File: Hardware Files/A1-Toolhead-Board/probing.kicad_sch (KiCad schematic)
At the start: 2 parts, among them J10 BL_PROBE, J9 ADXL345

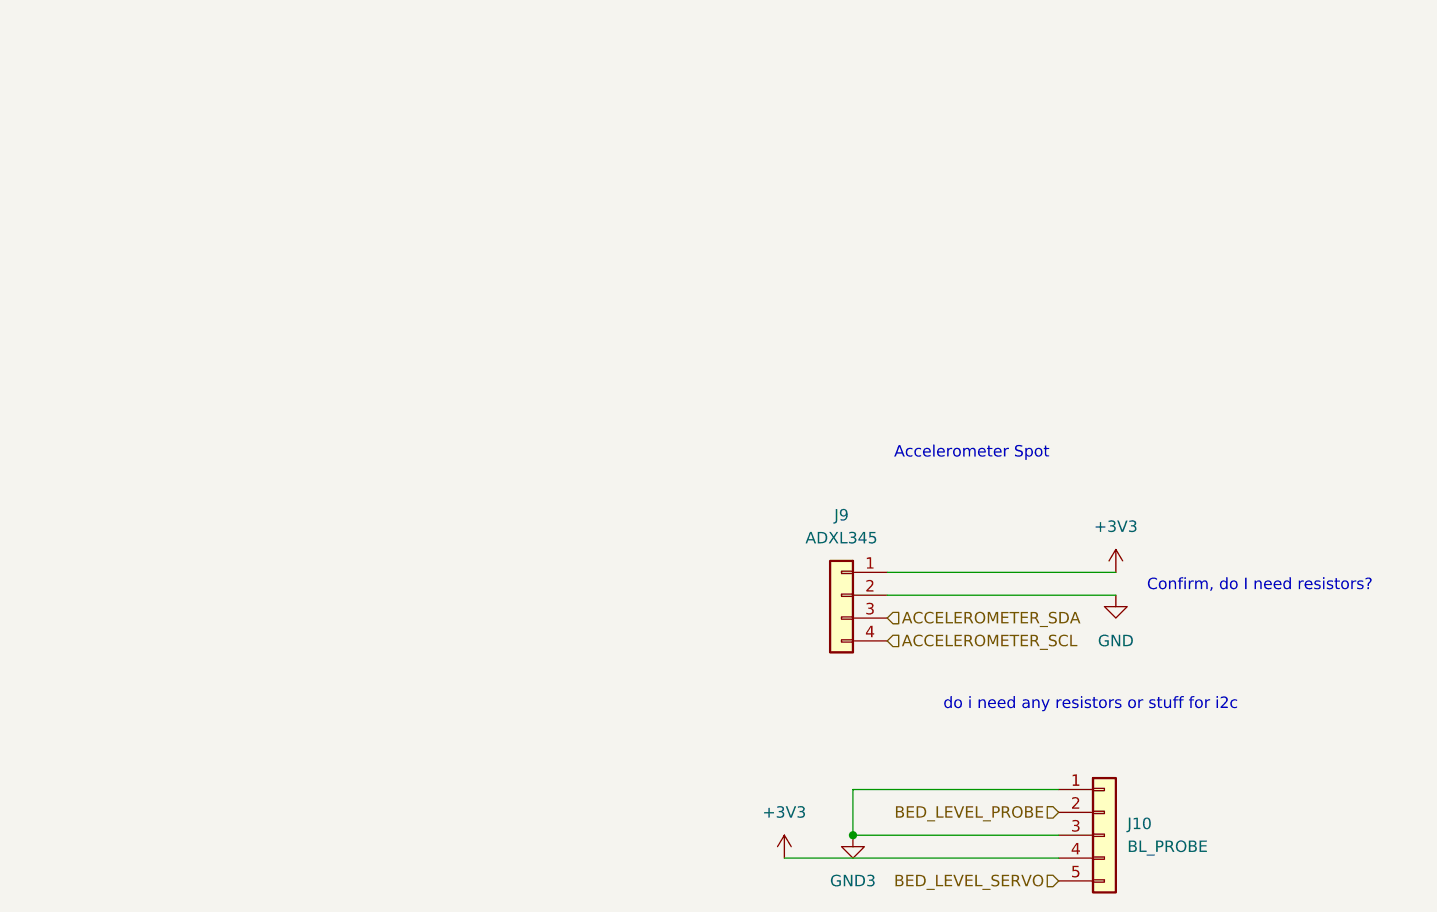
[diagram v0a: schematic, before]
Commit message: e
e
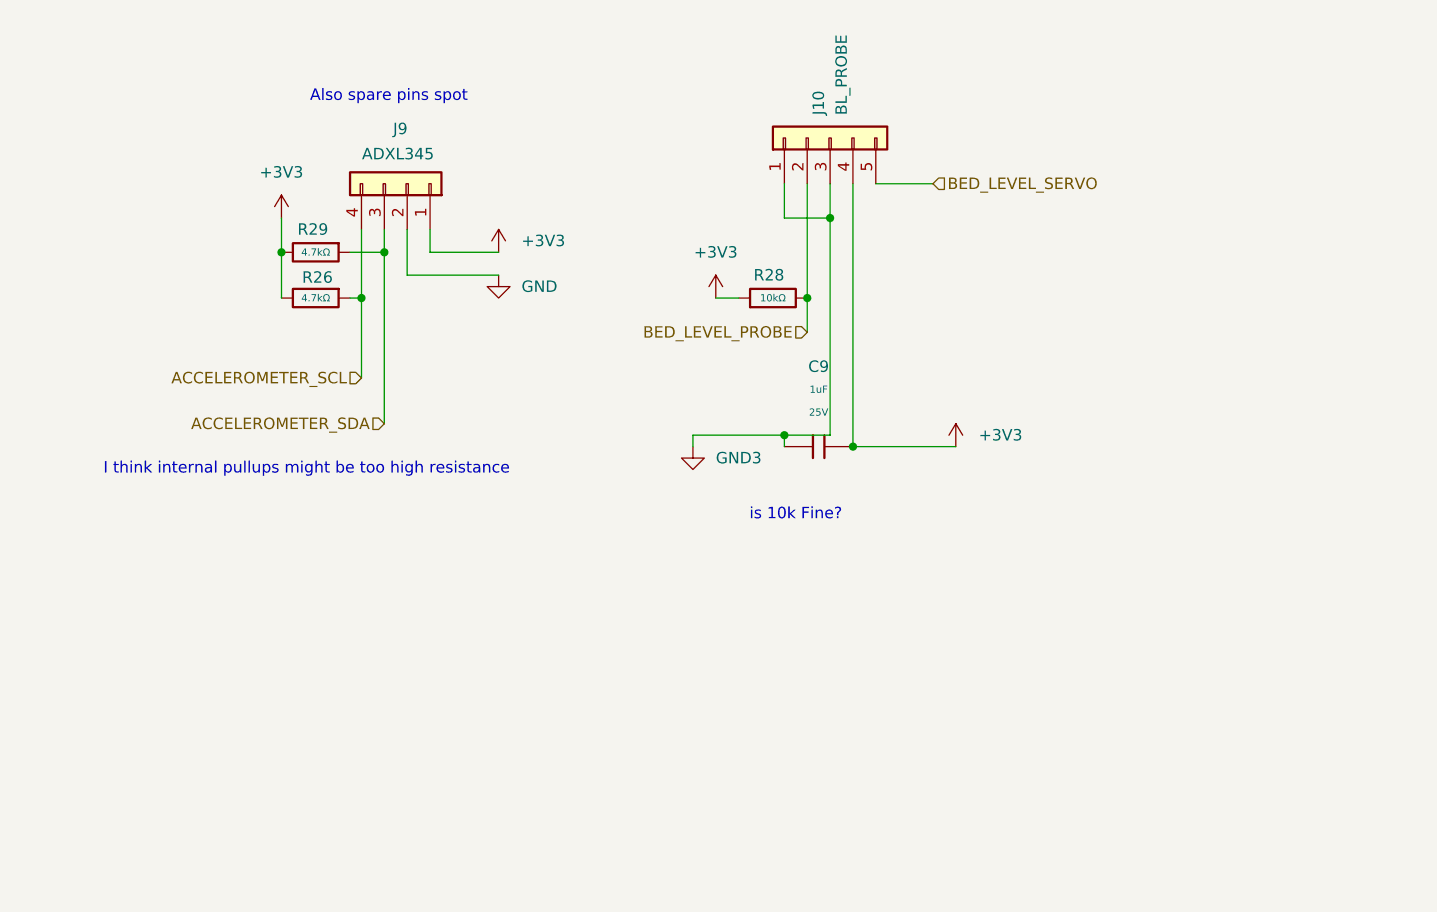
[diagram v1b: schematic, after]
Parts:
- added C9: 1uF, PCM_JLCPCB:C_0402, symbol PCM_JLCPCB-Capacitors:0402,1uF
- added R26, R29: 4.7kΩ, PCM_JLCPCB:R_0402, symbol PCM_JLCPCB-Resistors:0402,4.7kΩ
- added R28: 10kΩ, PCM_JLCPCB:R_0402, symbol PCM_JLCPCB-Resistors:0402,10kΩ
- J10: footprint Connector_JST:JST_XH_B5B-XH-A_1x05_P2.50mm_Vertical -> Connector_PinHeader_2.54mm:PinHeader_1x05_P2.54mm_Vertical
- J9: footprint Connector_JST:JST_XH_B4B-XH-A_1x04_P2.50mm_Vertical -> Connector_PinHeader_2.54mm:PinHeader_1x04_P2.54mm_Vertical
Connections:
- net +3V3: now also C9.2, R26.2, R28.1, R29.2
- net ACCELEROMETER_SCL: now also R26.1
- net ACCELEROMETER_SDA: now also R29.1
- net BED_LEVEL_PROBE: now also R28.2
- net GND3: now also C9.1
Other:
- note added: "Also spare pins spot"
- note added: "I think internal pullups might be too high resistance"
- note added: "is 10k Fine?"
- note removed: "Accelerometer Spot"
- note removed: "Confirm, do I need resistors?"
- note removed: "do i need any resistors or stuff for i2c"
- title: (none) -> Automatic Systems
- moved on the sheet: J10, J9

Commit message: e
e
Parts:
- J10: footprint Connector_PinHeader_2.54mm:PinHeader_1x05_P2.54mm_Vertical -> Connector_JST:JST_XH_B5B-XH-A_1x05_P2.50mm_Vertical
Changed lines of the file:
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@@
 			)
 		)
-		(property "Footprint" "Connector_PinHeader_2.54mm:PinHeader_1x05_P2.54mm_Vertical"
+		(property "Footprint" "Connector_JST:JST_XH_B5B-XH-A_1x05_P2.50mm_Vertical"
 			(at 125.73 40.64 0)
 			(hide yes)
